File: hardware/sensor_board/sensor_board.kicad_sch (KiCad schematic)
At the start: 22 parts, among them J1 CORTEX-SWD-6, J2 Molex PicoBlade 1x4, Q1 Q_NMOS_DGS, Q2 Q_NMOS_DGS, U1 ATSAMC21E17A, U2 TCAN332G, Y1 Crystal

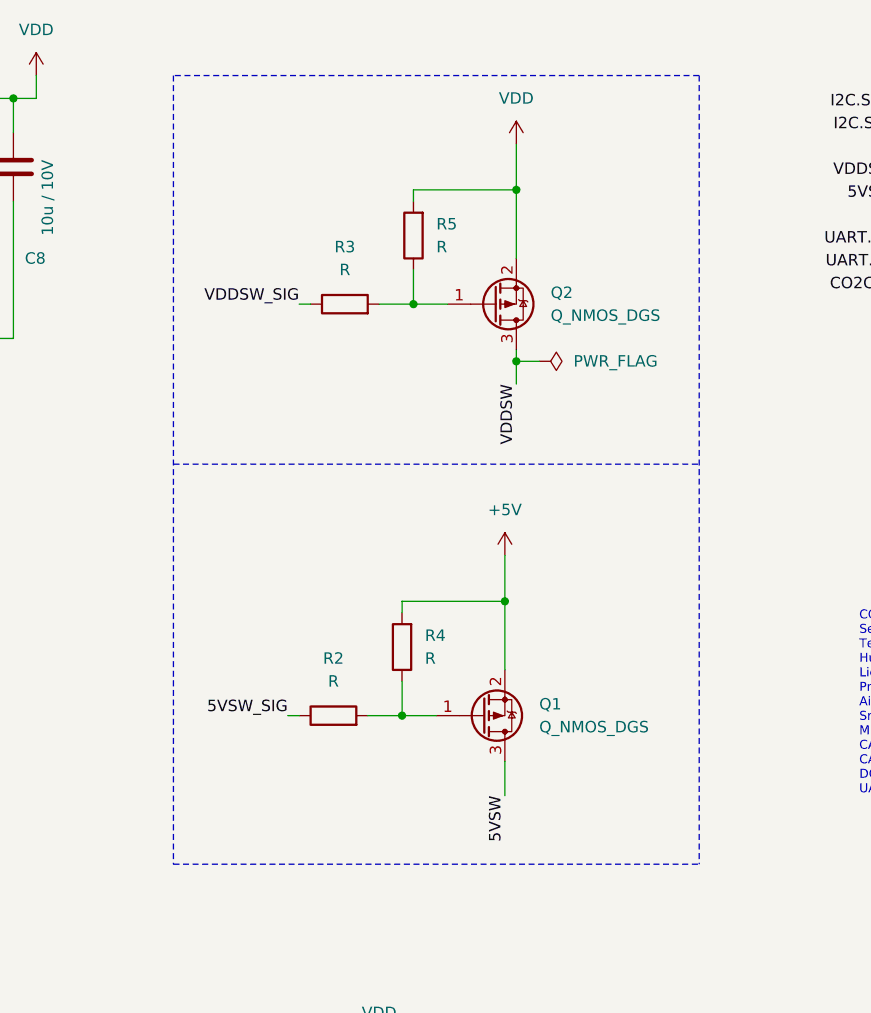
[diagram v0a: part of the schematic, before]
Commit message: did some stuff
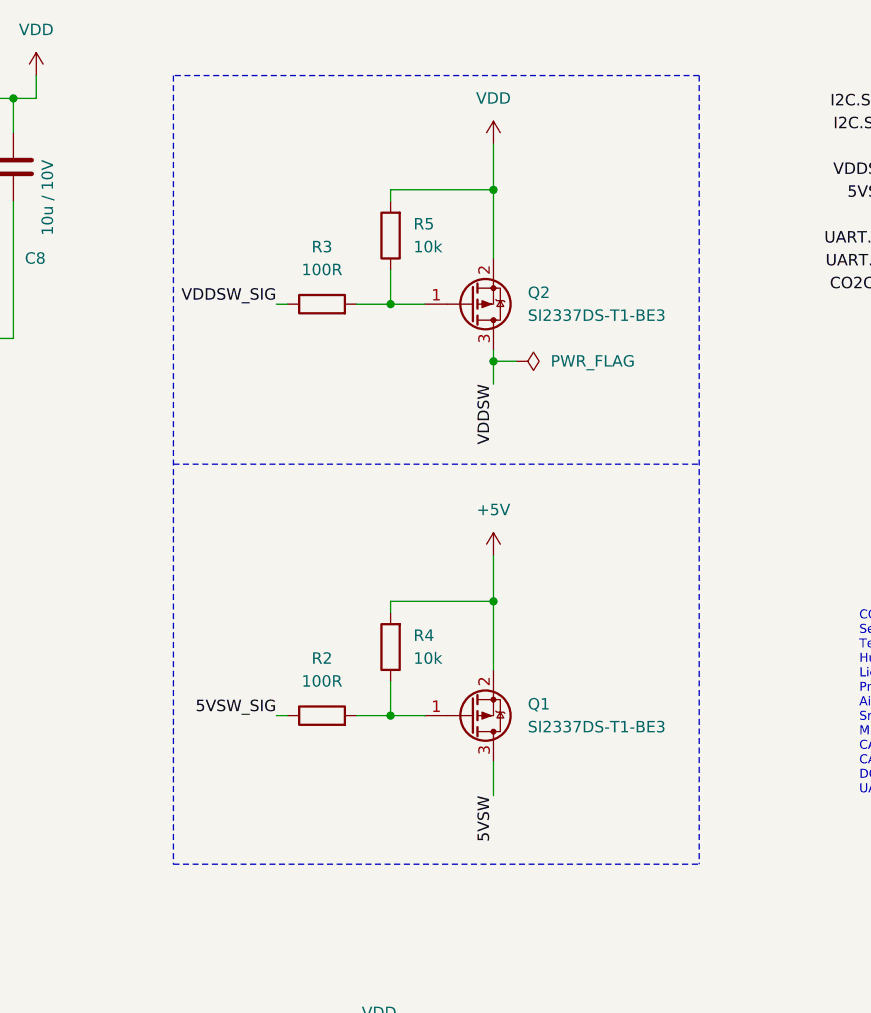
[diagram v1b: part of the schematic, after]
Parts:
- C1, C2, C3, C4, C5, C6, C7, C8: footprint (none) -> Capacitor_SMD:C_0603_1608Metric
- J2: footprint (none) -> Connector_Molex:Molex_PicoBlade_53261-0471_1x04-1MP_P1.25mm_Horizontal
- Q1, Q2: value Q_NMOS_DGS -> SI2337DS-T1-BE3; footprint (none) -> Package_TO_SOT_SMD:SOT-23
- R1: footprint (none) -> Resistor_SMD:R_0603_1608Metric
- R2, R3: value R -> 100R; footprint (none) -> Resistor_SMD:R_0603_1608Metric
- R4, R5: value R -> 10k; footprint (none) -> Resistor_SMD:R_0603_1608Metric
- R6: footprint (none) -> Resistor_SMD:R_1206_3216Metric
- U2: footprint (none) -> Package_SO:SOIC-8_3.9x4.9mm_P1.27mm
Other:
- moved on the sheet: Q1, Q2, R2, R3, R4, R5
